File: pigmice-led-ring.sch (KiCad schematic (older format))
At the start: 41 parts, among them J1 Conn_01x02_Female, J2 Conn_01x03_Female, U1 LMR62014XMF

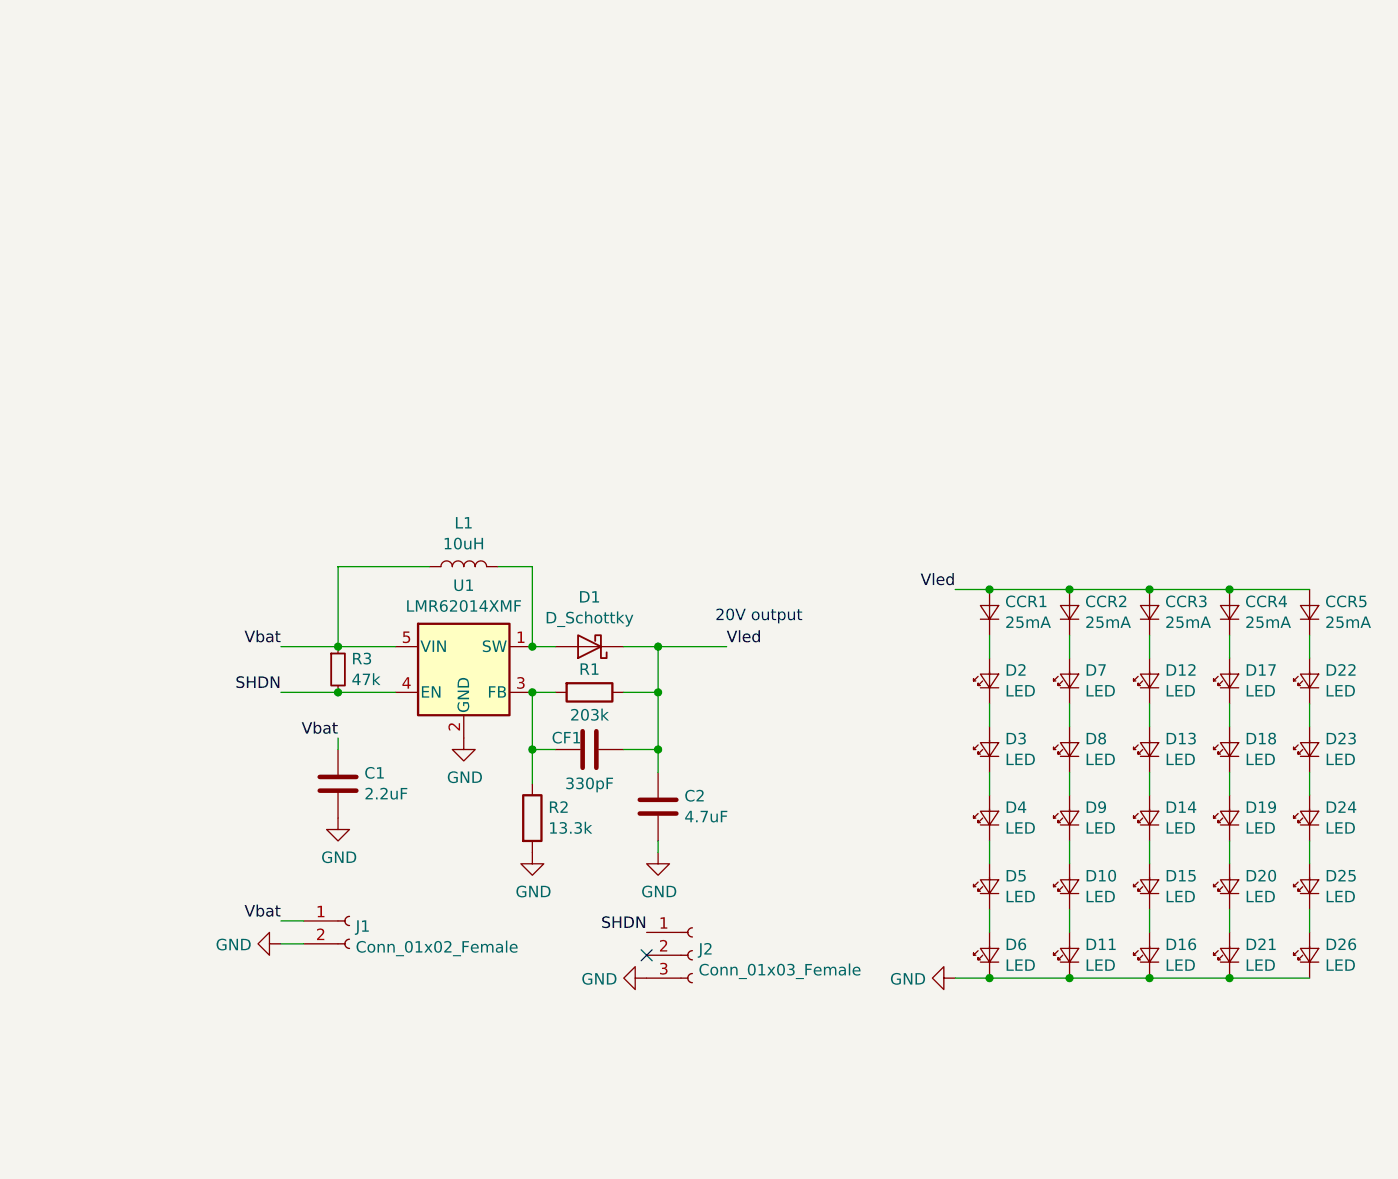
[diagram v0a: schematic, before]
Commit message: Add mini badge
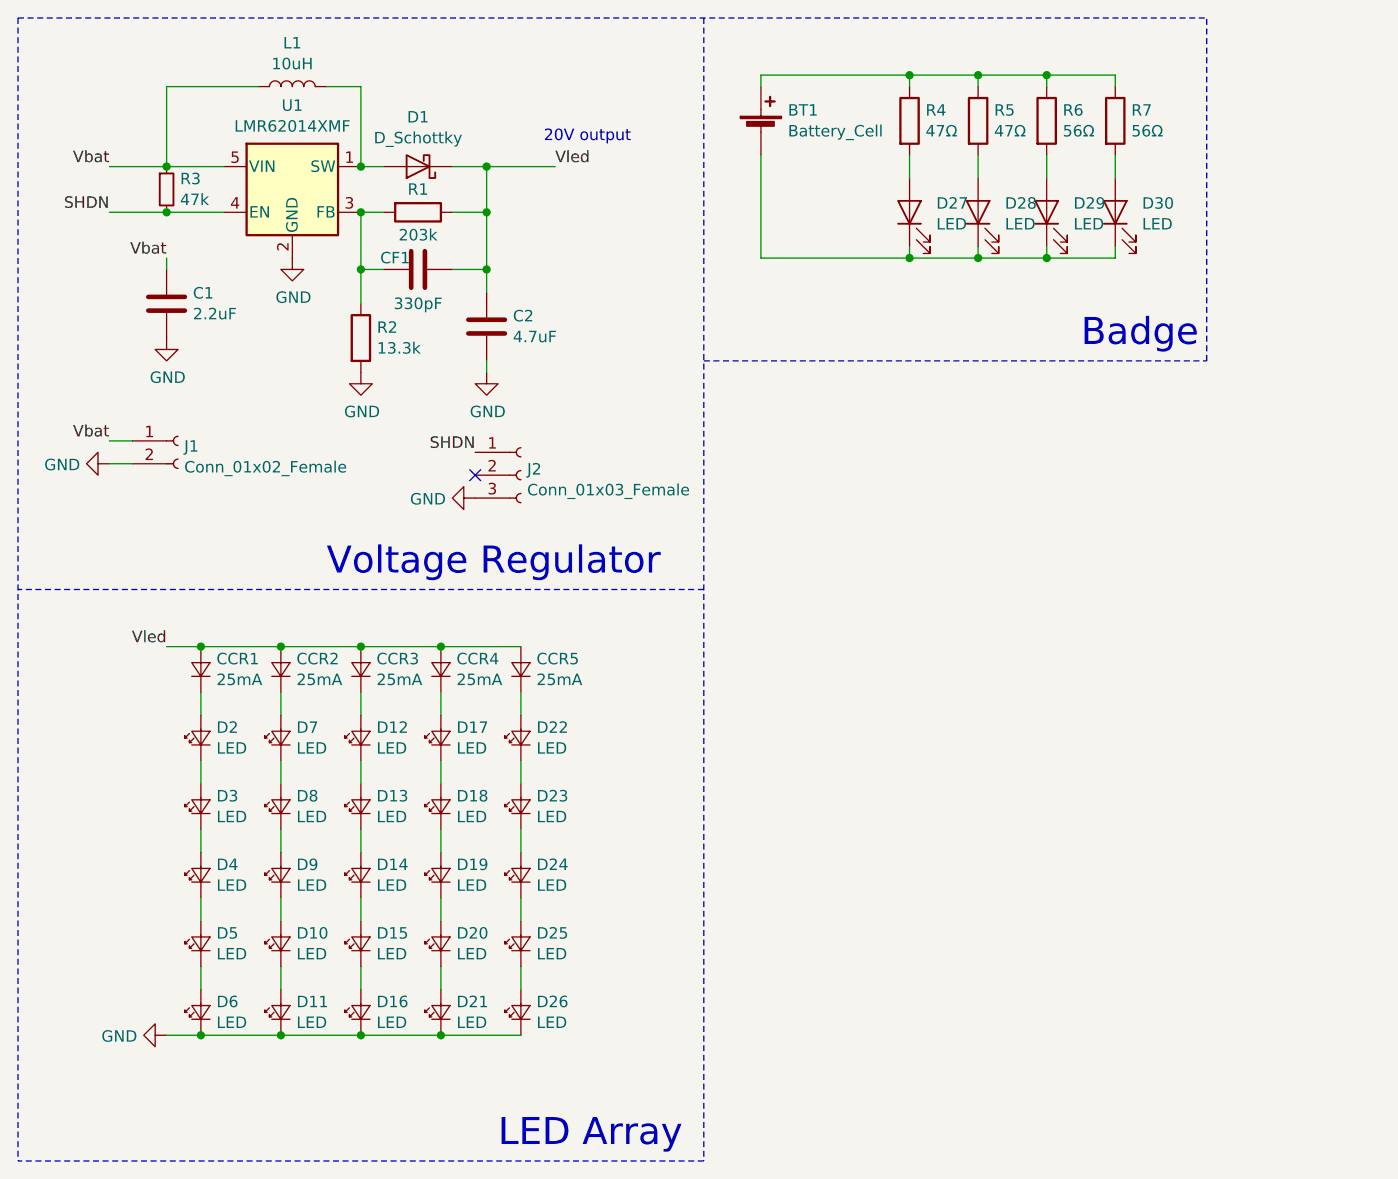
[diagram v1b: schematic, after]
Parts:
- added BT1: Battery_Cell, Battery:BatteryHolder_LINX_BAT-HLD-012-SMT, symbol Device:Battery_Cell
- added D27, D28, D29, D30: LED, LED_SMD:LED_0603_1608Metric, symbol Device:LED
- added R4, R5: 47Ω, Resistor_SMD:R_0603_1608Metric, symbol Device:R
- added R6, R7: 56Ω, Resistor_SMD:R_0603_1608Metric, symbol Device:R
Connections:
- new net: BT1.1 (+), R4.1, R5.1, R6.1, R7.1
- new net: BT1.2 (-), D27.1 (K), D28.1 (K), D29.1 (K), D30.1 (K)
- new net: D27.2 (A), R4.2
- new net: D28.2 (A), R5.2
- new net: D29.2 (A), R6.2
- new net: D30.2 (A), R7.2
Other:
- note added: "Badge"
- note added: "LED Array"
- note added: "Voltage Regulator"
- moved on the sheet: C1, C2, CCR1, CCR2, CCR3, CCR4, CCR5, CF1, D1, D10, D11, D12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
